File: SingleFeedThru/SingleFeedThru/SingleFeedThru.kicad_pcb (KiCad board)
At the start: 2 copper layers, 53 x 53 mm, 2 parts, among them J1 DB25_Male, J2 DB25_Male

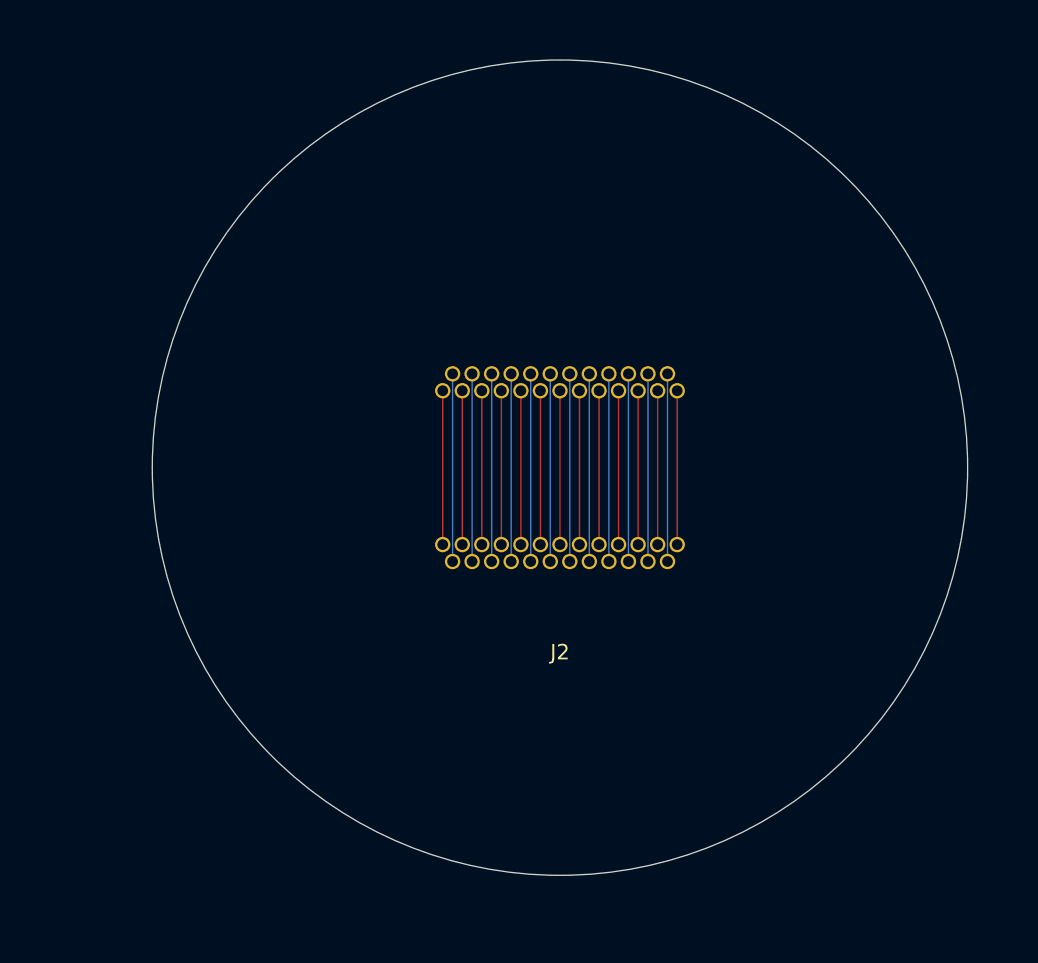
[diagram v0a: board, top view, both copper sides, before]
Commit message: Update Gerber
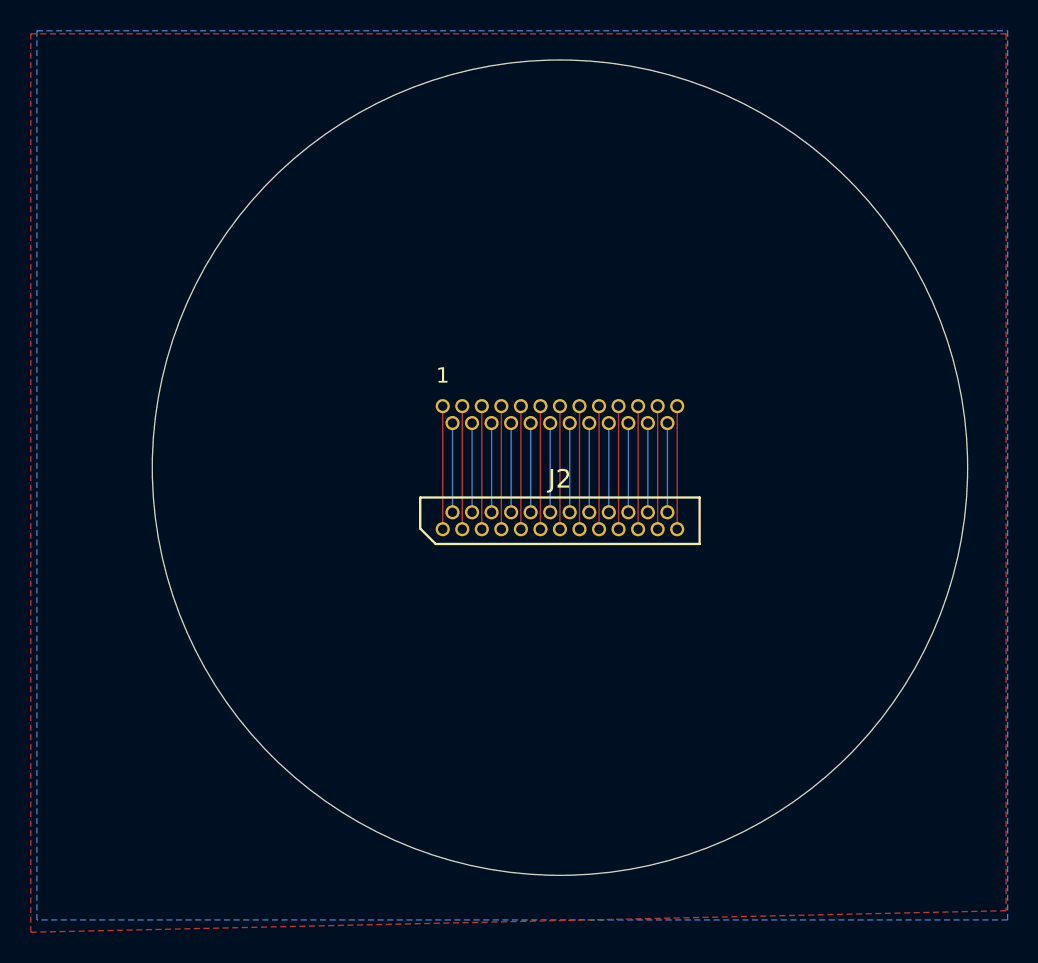
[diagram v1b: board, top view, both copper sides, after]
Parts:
- J1: footprint Connector:MicroD_25Pin_NorComp -> Connector:Norcomp-380-025-113L001-microd_Updated; moved to F.Cu
- J2: footprint Connector:MicroD_25Pin_NorComp -> Connector:Norcomp-380-025-113L001-microd_Updated; moved to B.Cu
- moved J1 7.78 mm to (0.00, -3.45)
- moved J2 7.78 mm to (0.00, 3.45)
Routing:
- net Net-(J1-Pad25): track 12.2 -> 5.80 mm
- net Net-(J1-Pad24): track 12.2 -> 5.80 mm
- net Net-(J1-Pad23): track 12.2 -> 5.80 mm
- net Net-(J1-Pad22): track 12.2 -> 5.80 mm
- net Net-(J1-Pad21): track 12.2 -> 5.80 mm
- net Net-(J1-Pad20): track 12.2 -> 5.80 mm
- net Net-(J1-Pad19): track 12.2 -> 5.80 mm
- net Net-(J1-Pad18): track 12.2 -> 5.80 mm
- net Net-(J1-Pad17): track 12.2 -> 5.80 mm
- net Net-(J1-Pad16): track 12.2 -> 5.80 mm
- net Net-(J1-Pad15): track 12.2 -> 5.80 mm
- net Net-(J1-Pad14): track 12.2 -> 5.80 mm
- net Net-(J1-Pad9): track 10.0 -> 8.00 mm
- net Net-(J1-Pad8): track 10.0 -> 8.00 mm
- net Net-(J1-Pad7): track 10.0 -> 8.00 mm
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- added copper zone on B.Cu, net (none)
- added copper zone on F.Cu, net (none)
